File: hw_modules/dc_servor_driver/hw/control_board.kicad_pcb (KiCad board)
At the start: 2 copper layers, 66 x 22.9 mm, 33 parts, among them P1 CONN_02X03, P2 CONN_01X06, P3 CONN_01X03, P4 CONN_02X03, Q1 BSS138, Q4 BSS138, Q5 BSS138, Q6 BSS138, Q7 BSS138, U1 STM32F030F4, U2 APE8865N-33-HF-3, Y1 8Mhz

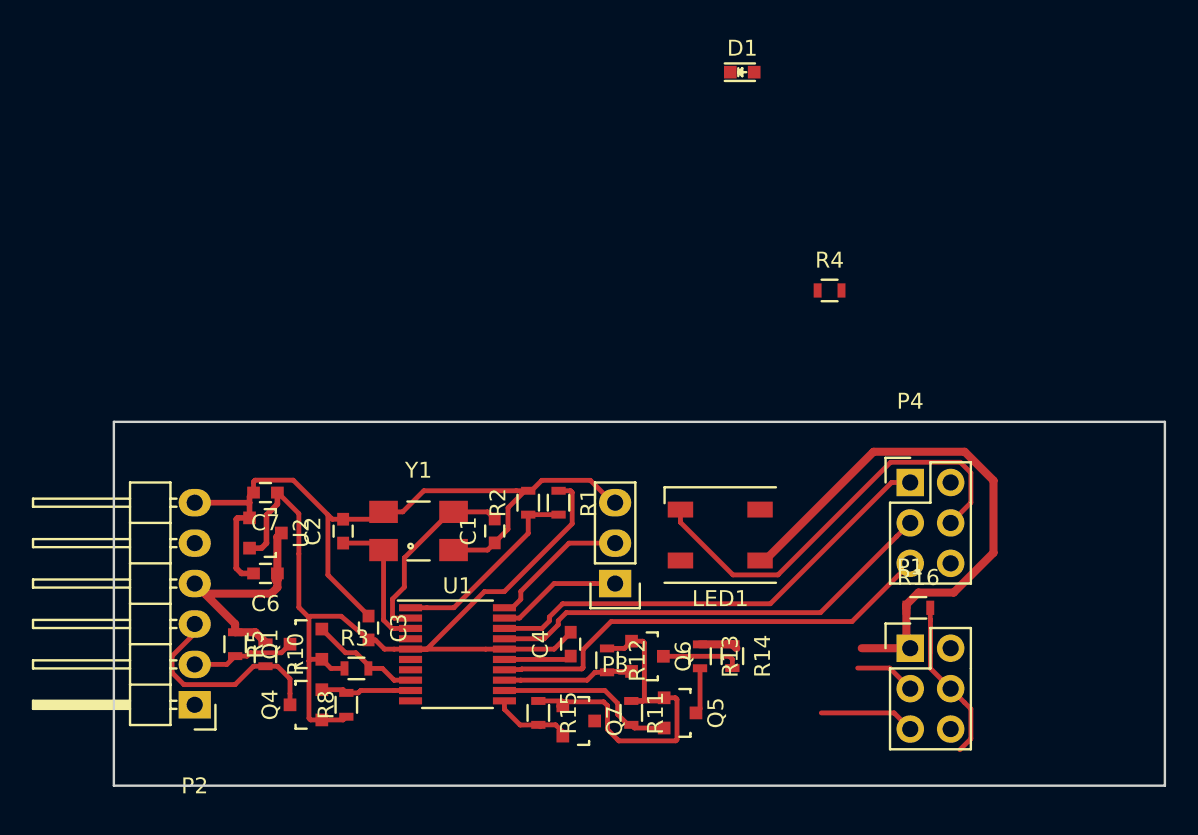
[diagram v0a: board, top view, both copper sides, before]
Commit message: Firt verision of dc_servo_driver board
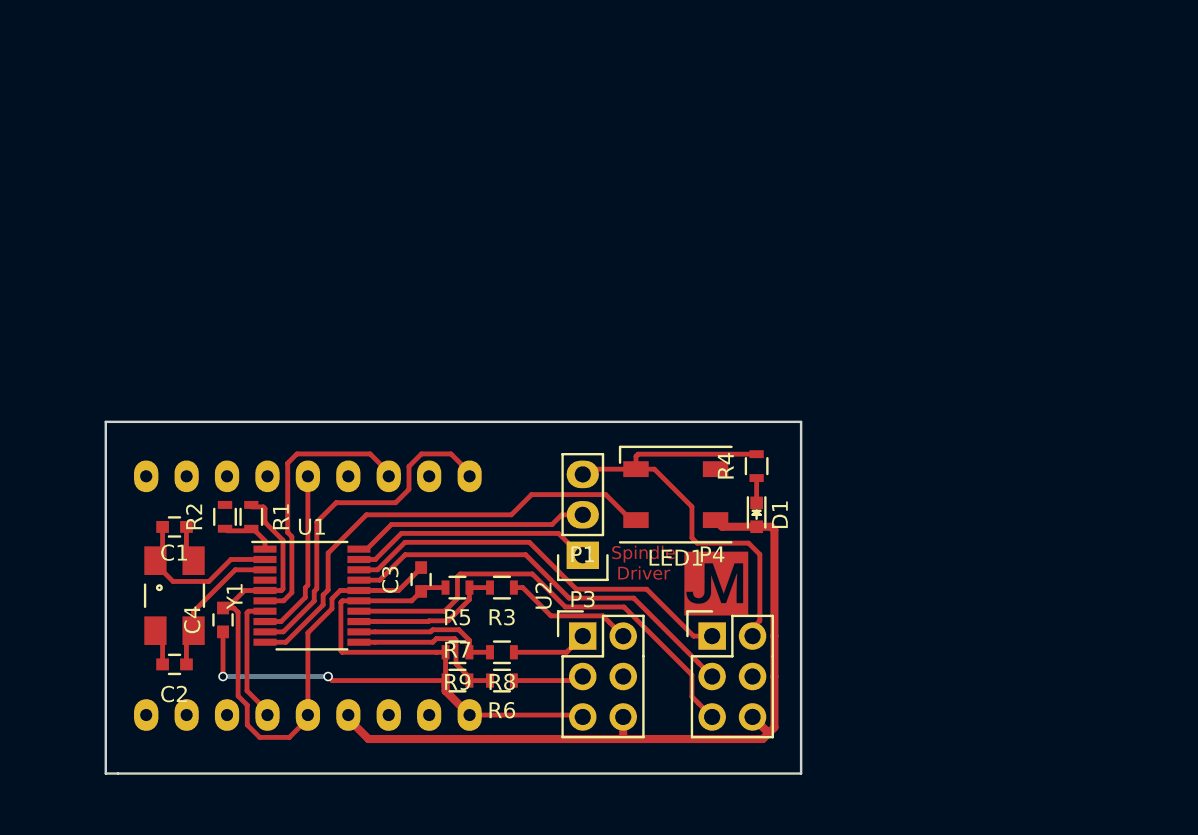
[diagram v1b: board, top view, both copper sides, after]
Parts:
- removed C6: 470n, Capacitors_SMD:C_0603
- removed C7: 100n, Capacitors_SMD:C_0603
- removed P2: CONN_01X06, Pin_Headers:Pin_Header_Angled_1x06
- removed Q1, Q4, Q5, Q6, Q7: BSS138, TO_SOT_Packages_SMD:SOT-23
- removed R10, R11, R12, R13, R14, R15, R16: 10k, Resistors_SMD:R_0603
- added G***: LOGO, yaqwsx:JM_4, F.Cu at (159.8, 96.5)
- added R6: 10k, Resistors_SMD:R_0603, F.Cu at (146.3, 102.6)
- added R7: 20k, Resistors_SMD:R_0603, F.Cu at (143.5, 102.6)
- added R9: 20k, Resistors_SMD:R_0603, F.Cu at (143.5, 100.8)
- R5: value 10k -> 20k
- U2: value APE8865N-33-HF-3 -> FDI_Module_Half; footprint TO_SOT_Packages_SMD:SOT-23 -> yaqwsx:FTDI_Half
- Y1: value 8Mhz -> Crystal_Four_Pin
- moved D1 27.8 mm to (162.3, 92.2), turned to 270 degrees
- moved C4 21.9 mm to (128.8, 98.8)
- moved P1 20.6 mm to (151.4, 99.8)
- moved C1 20.1 mm to (125.7, 93.0), turned to 180 degrees
- moved R1 19.3 mm to (130.6, 92.3)
- moved R2 19.1 mm to (128.9, 92.3)
- moved Y1 15.9 mm to (125.7, 97.3), turned to 270 degrees
- moved P4 15.8 mm to (159.5, 99.8)
- moved R5 14.4 mm to (143.5, 96.8), turned to 180 degrees
- moved C2 13.5 mm to (125.7, 101.6), turned to 180 degrees
- moved R4 12.0 mm to (162.3, 89.1), turned to 90 degrees
- moved R3 10.5 mm to (146.3, 96.8), turned to 180 degrees
- moved R8 10.3 mm to (146.3, 100.8), turned to 180 degrees
- moved U1 9.86 mm to (134.4, 97.3)
- moved U2 8.46 mm to (124.0, 97.3), turned to 90 degrees
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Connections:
- P1 pad 1: +5V -> ENCODER_A_5
- P1 pad 2: GND -> ENCODER_B_5
- P1 pad 3: ENCODER_B_5 -> ENCODER_INDEX_5
- P1 pad 4: ENCODER_INDEX_5 -> (no net)
- P1 pad 5: ENCODER_A_5 -> GND
- P1 pad 6: (no net) -> +5V
- P4 pad 2: +3V3 -> GND
- P4 pad 4: GND -> (no net)
- P4 pad 6: (no net) -> +5V
- R3 pad 1: +3V3 -> ENCODER_B_5
- R3 pad 2: UART_TX_3.3 -> ENCODER_B_3.3
- R5 pad 1: +5V -> ENCODER_B_3.3
- R5 pad 2: UART_TX_5 -> GND
- R8 pad 1: +3V3 -> ENCODER_A_5
- R8 pad 2: UART_RX_3.3 -> ENCODER_A_3.3
- U1 pad 6: (no net) -> UART_CTS
- U1 pad 7: (no net) -> UART_RTS
- U1 pad 8: UART_TX_3.3 -> UART_TX
- U1 pad 9: UART_RX_3.3 -> UART_RX
- U2 pad 1: GND -> (no net)
- U2 pad 2: +3V3 -> (no net)
- U2 pad 3: +5V -> (no net)
- Y1 pad 1: Net-(C2-Pad1) -> Net-(C1-Pad2)
- Y1 pad 3: Net-(C1-Pad2) -> Net-(C2-Pad1)
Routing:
- net +3V3: track 82.4 -> 38.0 mm
- net STATE_LED: track 0.00 -> 29.5 mm
- net UART_RX: track 0.00 -> 21.9 mm
- net UART_CTS: track 0.00 -> 17.5 mm
- net UART_RX_5: track 14.0 -> 0.00 mm
- net UART_TX: track 0.00 -> 10.8 mm
- net /boot_sel: track 12.4 -> 3.17 mm
- net UART_RTS: track 0.00 -> 8.13 mm
- net SWDIO: track 7.85 -> 15.7 mm
- net ENCODER_INDEX_5: track 11.7 -> 4.44 mm
- net UART_TX_3.3: track 7.02 -> 0.00 mm
- net +5V: track 53.7 -> 47.0 mm
- net UART_TX_5: track 6.67 -> 0.00 mm
- net SWCLK: track 8.93 -> 15.0 mm
- net UART_RX_3.3: track 6.00 -> 0.00 mm
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- added copper zone on F.Cu, net GND
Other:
- board size 66 x 22.9 mm -> 43.7 x 22.1 mm
- net class power: via_dia 0.6 -> 1.5; via_drill 0.4 -> 0.8
- rule trace_min: 0.2 -> 0.007874
- rule via_min_size: 0.4 -> 0.015748
- board text added: "Spindle Driver"
